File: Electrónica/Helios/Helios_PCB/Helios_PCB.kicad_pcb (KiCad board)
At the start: 2 copper layers, 35 x 30.3 mm, 12 parts, among them J0 Connector J0, J1 Connector J1, U0 OPA2380, U1 OPA2380

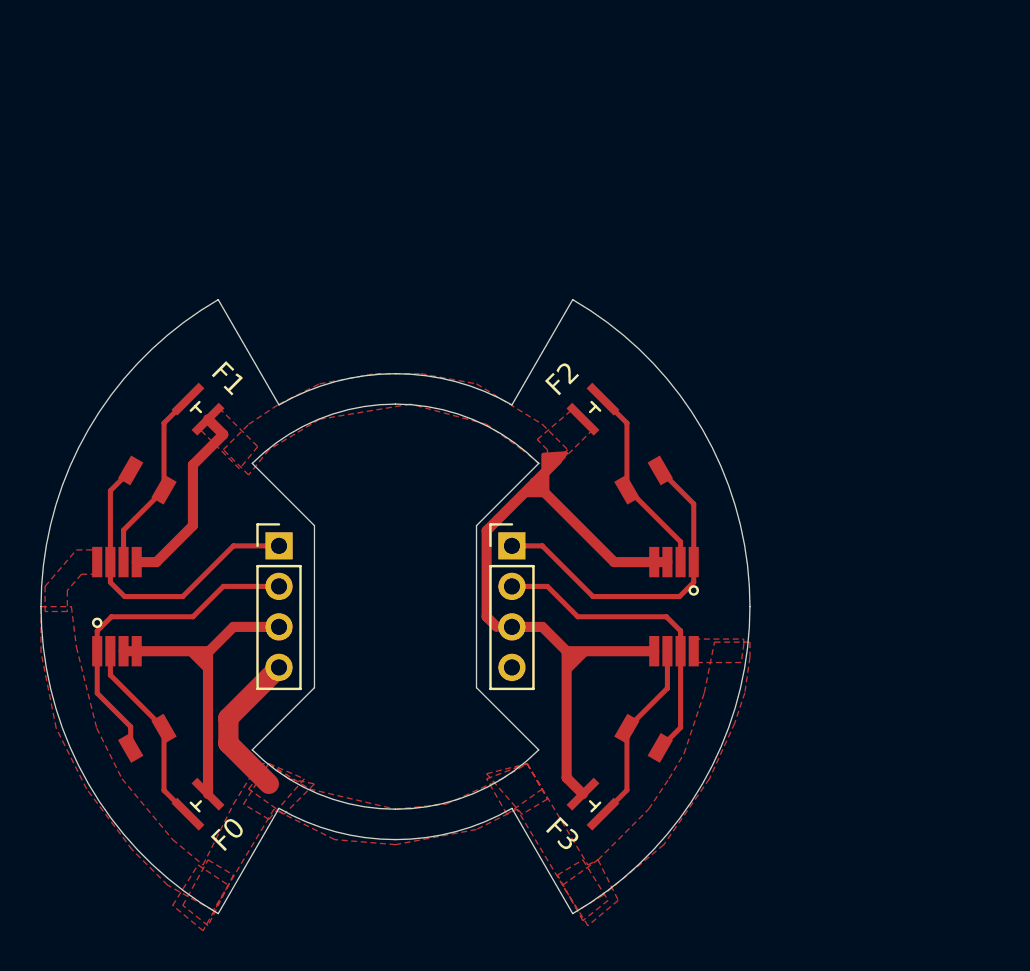
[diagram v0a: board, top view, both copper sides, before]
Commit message: Revert "Revert "Helios: Bot Layer Sch. (LEDs)""
This reverts commit 5c5999d2bbe18ce28315539fce76e1635c27d7e8.
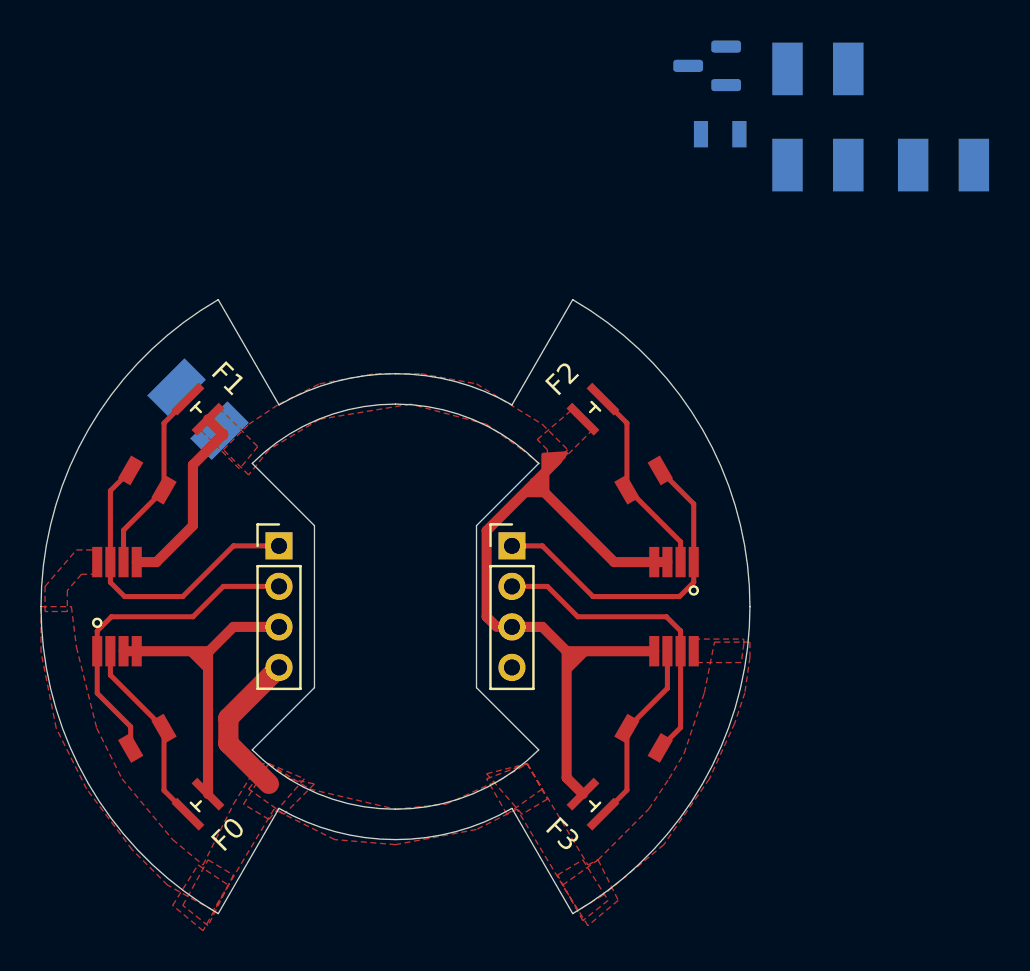
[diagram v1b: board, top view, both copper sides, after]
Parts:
- added D0: LED, LED_SMD:LED_PLCC-2, B.Cu at (170.9, 78.2)
- added D1: LED, LED_SMD:LED_PLCC-2, B.Cu at (140.2, 90.2)
- added D2: LED, LED_SMD:LED_PLCC-2, B.Cu at (177.1, 78.2)
- added D3: LED, LED_SMD:LED_PLCC-2, B.Cu at (170.9, 73.5)
- added Q1: AO3400A, Package_TO_SOT_SMD:SOT-23, B.Cu at (165.4, 73.3)
- added R5: R, Helios:RS_0805, B.Cu at (166.0, 76.7)

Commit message: Revert "Helios: Bot Layer Sch. (LEDs)"
This reverts commit dca8e3bb9b15b9e1c7b2acfc811398ae5ce91dcf.
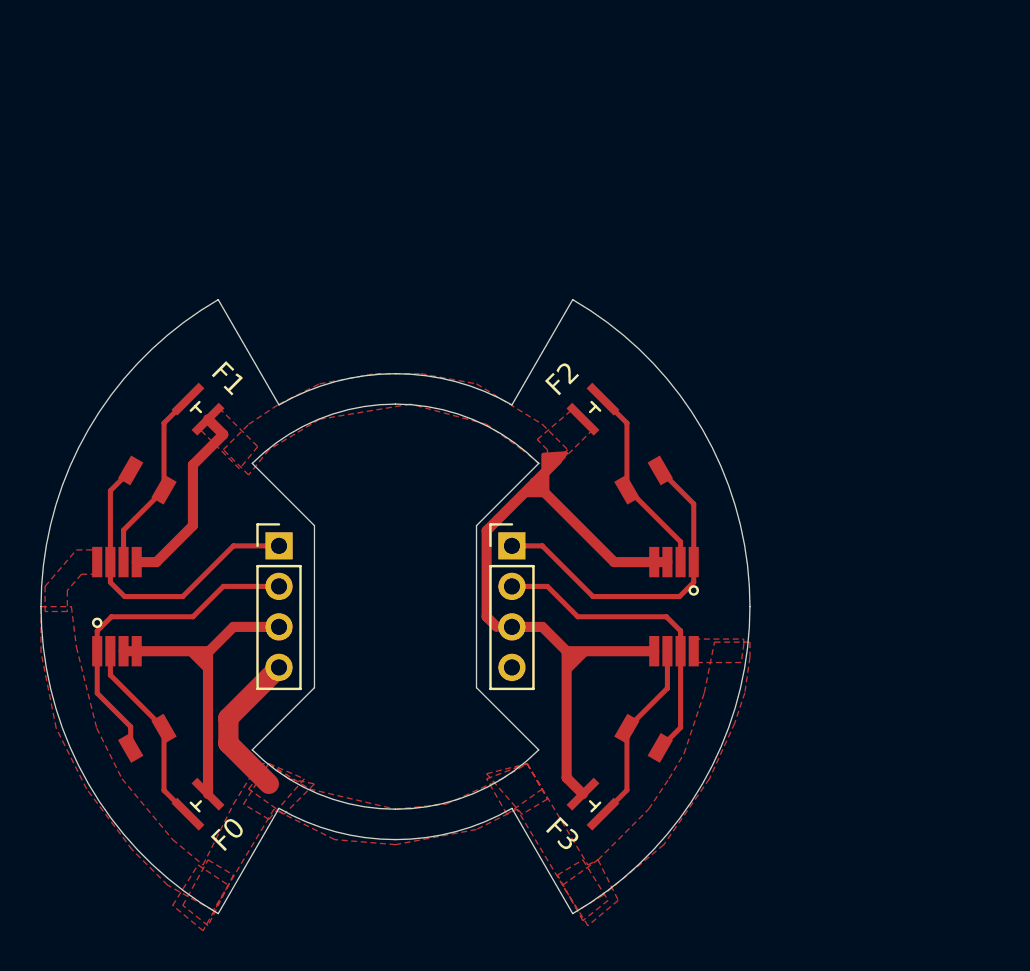
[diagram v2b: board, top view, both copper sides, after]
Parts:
- removed D0, D1, D2, D3: LED, LED_SMD:LED_PLCC-2
- removed Q1: AO3400A, Package_TO_SOT_SMD:SOT-23
- removed R5: R, Helios:RS_0805
